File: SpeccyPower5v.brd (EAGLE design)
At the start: 112.1 x 37.5 mm, 63 parts, among them T1 TRANS_ER29

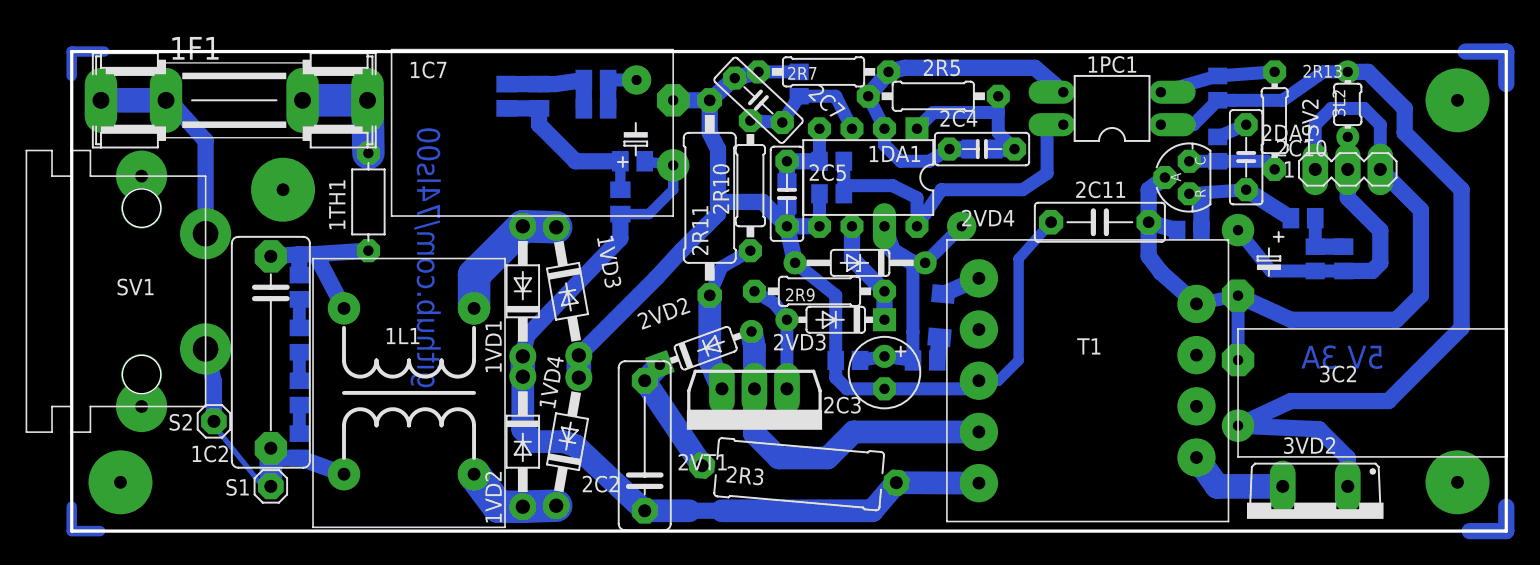
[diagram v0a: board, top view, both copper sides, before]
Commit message: ..
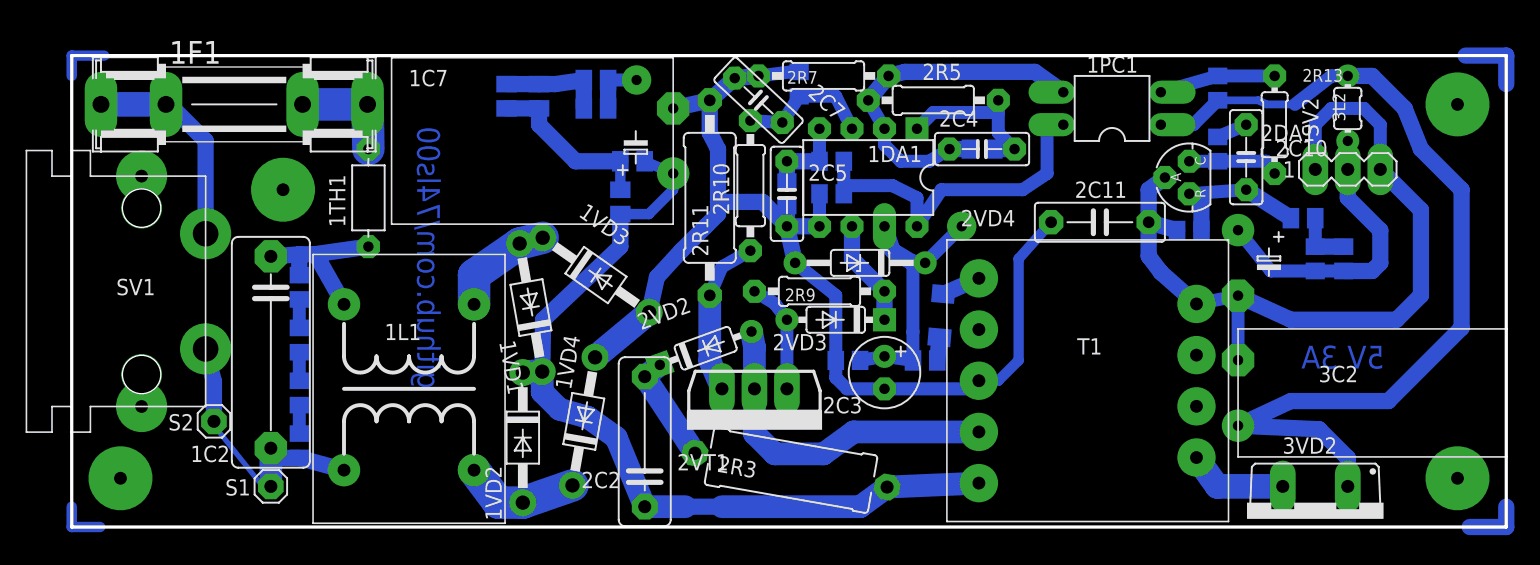
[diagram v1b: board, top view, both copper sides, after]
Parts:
- moved 1VD3 2.56 mm to (54.3, 55.6), turned to 325 degrees
- moved 1VD4 2.03 mm to (53.3, 44.1)
- moved 1VD1 1.42 mm to (49.2, 53.0), turned to 100 degrees
- moved 2R3 0.71 mm to (69.5, 40.3), turned to 350 degrees
- moved 1C7 0.63 mm to (60.3, 66.0)
- moved 1F1 0.32 mm to (26.0, 68.9)
- moved 1L1 0.32 mm to (39.7, 46.7)
- moved 2C2 0.32 mm to (58.1, 42.5)
- moved 1TH1 0.32 mm to (36.5, 61.6)
- moved 1VD2 0.32 mm to (48.6, 42.9)
- moved 2R13 0.32 mm to (107.3, 67.3)
- moved 2R5 0.32 mm to (80.6, 69.2)
- moved 2R7 0.32 mm to (72.1, 71.1)
- moved 3L2 0.32 mm to (113.0, 68.6)
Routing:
- net N$1: track 10.6 -> 8.47 mm
- net -IN: track 90.4 -> 88.4 mm
- net +IN: track 68.0 -> 66.0 mm
- net N$44: track 7.69 -> 9.19 mm
- net N$30: track 9.72 -> 8.65 mm
- net N$45: track 9.14 -> 8.51 mm
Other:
- board size 112.1 x 37.5 mm -> 112.1 x 36.8 mm
